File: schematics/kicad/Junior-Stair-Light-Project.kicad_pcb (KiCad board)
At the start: 2 copper layers, 90 x 90 mm, 107 parts, among them J1 12V Eingang, J2 Conn_01x06, J3 CONN_01X03, J4 CONN_01X03, J5 Conn_01x06, J6 Conn_01x06, T10_1 BC337, T10_2 BC327, T11_1 BC337, T11_2 BC327, T12_1 BC337, T12_2 BC327, T13_1 BC337, T13_2 BC327, T14_1 BC337, T14_2 BC327, T15_1 BC337, T15_2 BC327, T16_1 BC337, T16_2 BC327, T17_1 BC337, T17_2 BC327, T18_1 BC337, T18_2 BC327, T1_1 BC337, T1_2 BC327, T2_1 BC337, T2_2 BC327, T3_1 BC337, T3_2 BC327, T4_1 BC337, T4_2 BC327, T5_1 BC337, T5_2 BC327, T6_1 BC337, T6_2 BC327, T7_1 BC337, T7_2 BC327, T8_1 BC337, T8_2 BC327, T9_1 BC337, T9_2 BC327, U1 L4940V5, U2 Arduino_Nano

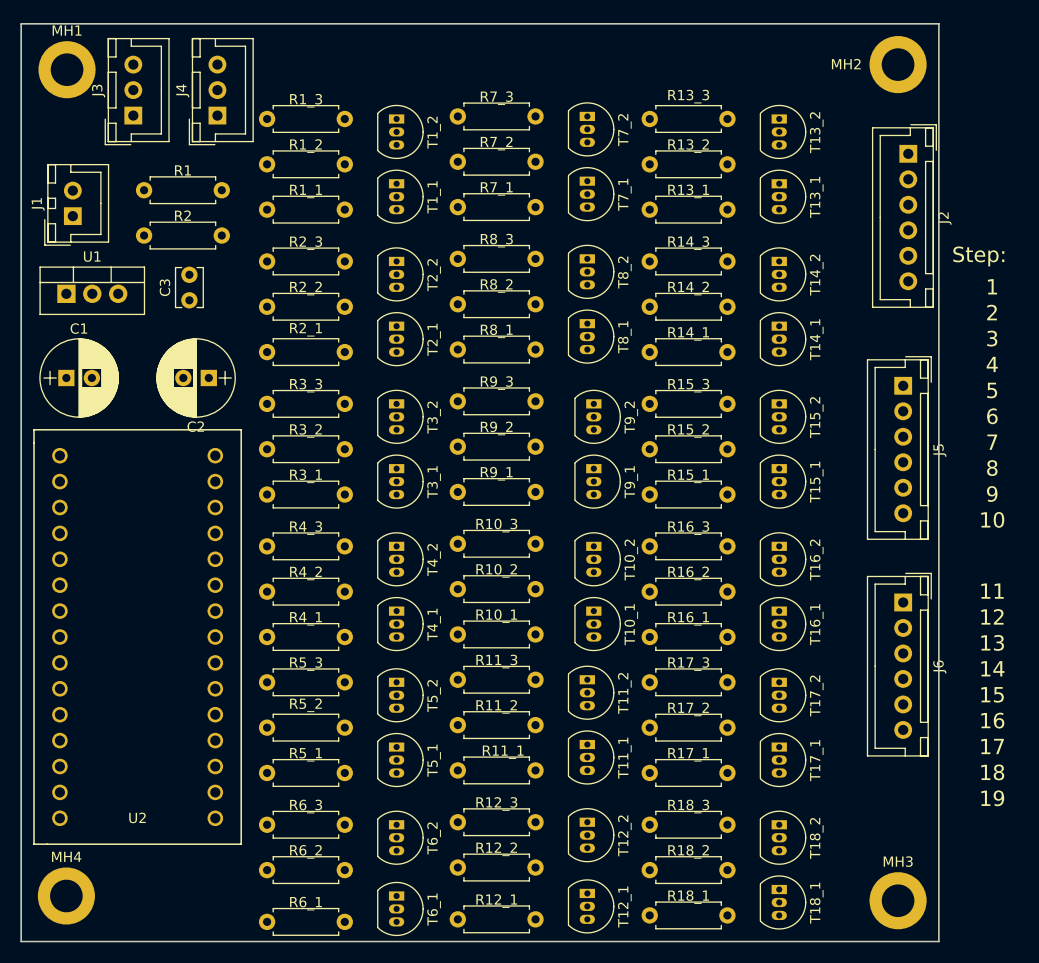
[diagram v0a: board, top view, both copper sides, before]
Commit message: Updates, updates, updates
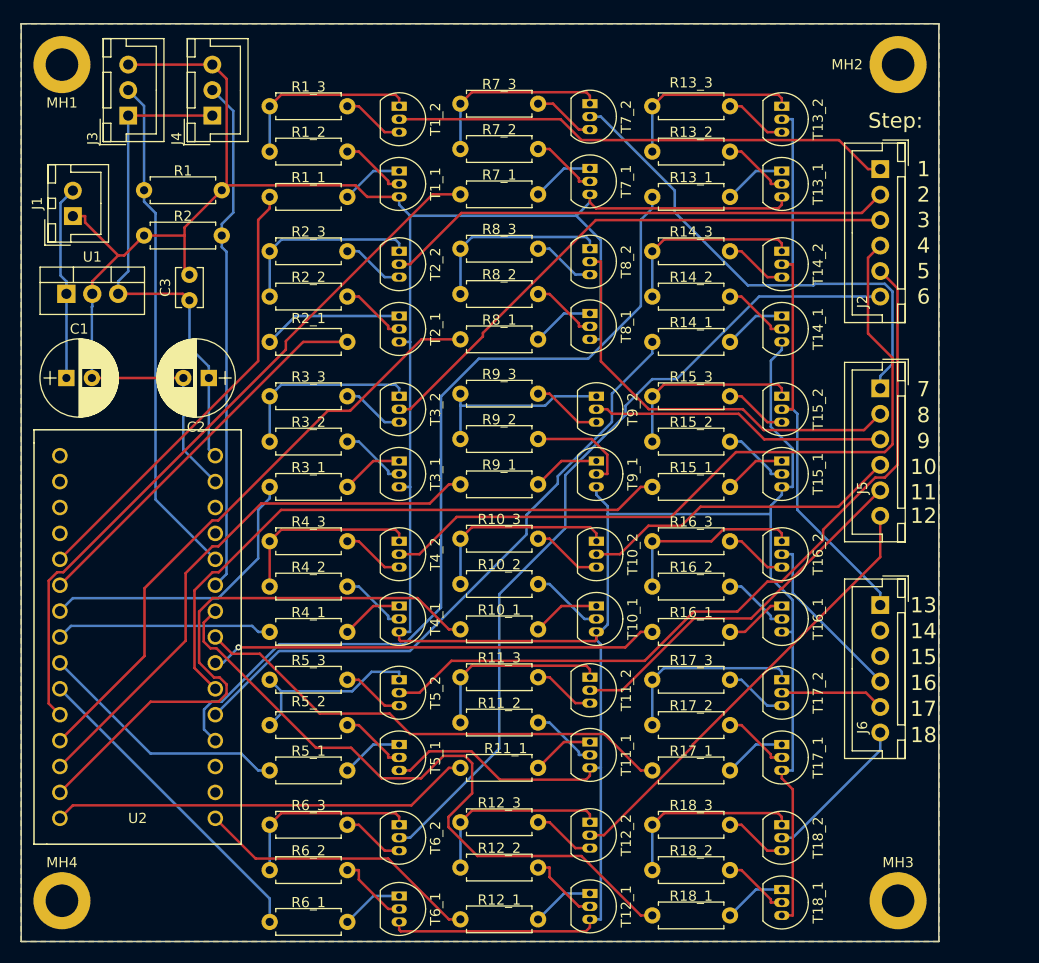
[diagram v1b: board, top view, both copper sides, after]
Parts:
- moved J2 3.13 mm to (194.8, 81.8)
- moved J5 2.26 mm to (194.8, 103.2)
- moved J6 2.26 mm to (194.8, 124.5)
- moved R13_1 1.27 mm to (180.0, 84.5)
- moved R13_2 1.27 mm to (172.4, 80.0)
- moved R13_3 1.27 mm to (172.4, 75.6)
- moved R1_1 1.27 mm to (142.5, 84.5)
- moved R1_2 1.27 mm to (134.9, 80.0)
- moved R1_3 1.27 mm to (134.9, 75.6)
- moved R7_1 1.27 mm to (161.2, 84.2)
- moved R7_2 1.27 mm to (153.6, 79.8)
- moved R7_3 1.27 mm to (153.6, 75.3)
- moved T13_1 1.27 mm to (185.1, 81.9)
- moved T13_2 1.27 mm to (185.1, 75.6)
- moved T1_1 1.27 mm to (147.6, 81.9)
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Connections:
- R1 pad 1: +5V -> GND
- R2 pad 1: +5V -> GND
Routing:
- net GND: track 0.00 -> 385.0 mm
- net Step13_a: track 0.00 -> 86.0 mm
- net Step6: track 0.00 -> 81.6 mm
- net Step5: track 0.00 -> 78.4 mm
- net Step4: track 0.00 -> 73.8 mm
- net Step7_a: track 0.00 -> 70.2 mm
- net Step18_a: track 0.00 -> 67.4 mm
- net Step14_a: track 0.00 -> 61.8 mm
- net Step15_a: track 0.00 -> 59.6 mm
- net Step8_a: track 0.00 -> 59.5 mm
- net Step10_a: track 0.00 -> 57.3 mm
- net Step13: track 0.00 -> 56.6 mm
- net Step3: track 0.00 -> 55.1 mm
- net Step9_a: track 0.00 -> 54.6 mm
- net Net-(J4-Pad2): track 0.00 -> 50.5 mm
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- added copper zone on B.Cu, net GND
- added copper zone on F.Cu, net GND
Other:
- board text removed: "19"
